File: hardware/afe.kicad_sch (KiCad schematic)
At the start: 53 parts, among them J2 DNP, J3 DNP, J4 Conn_01x19_Male, U2 BQ76200PW, U3 LTC6813-1

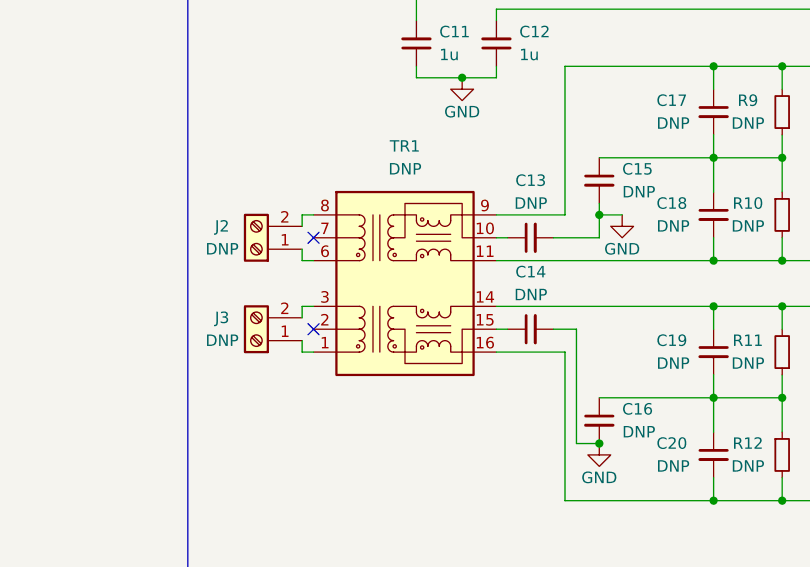
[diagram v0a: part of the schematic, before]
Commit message: Update design to KiCAD v7
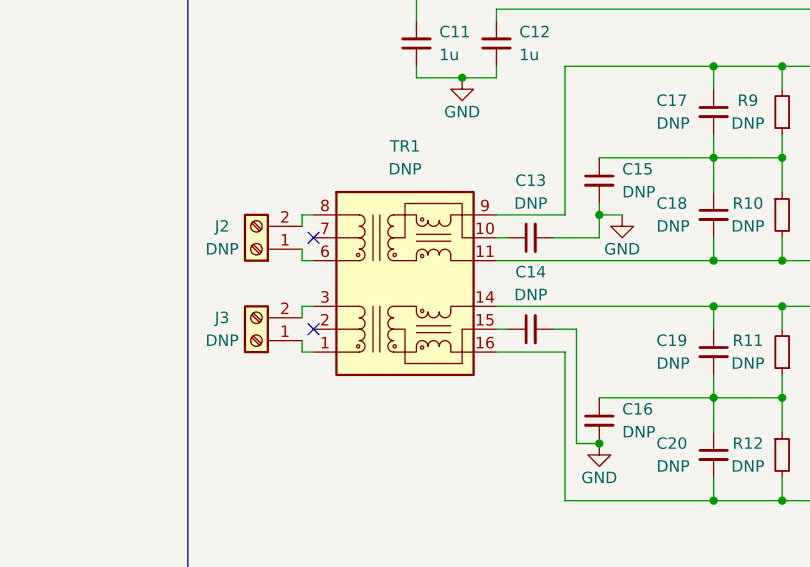
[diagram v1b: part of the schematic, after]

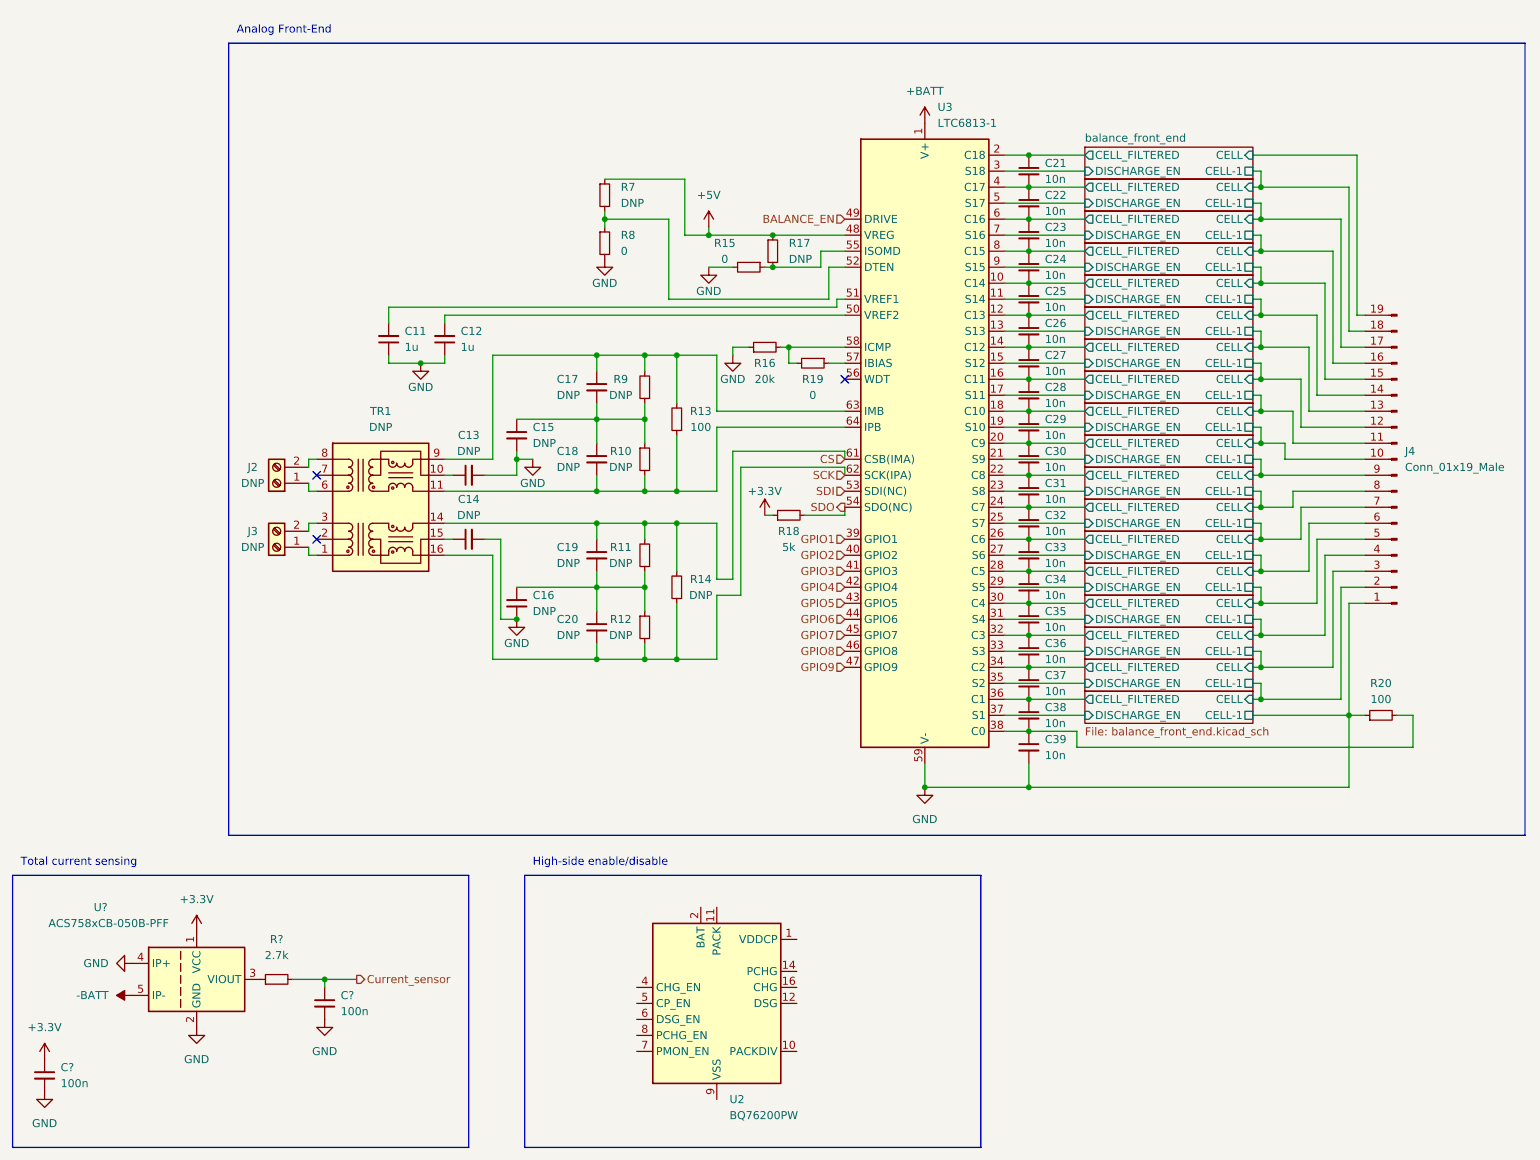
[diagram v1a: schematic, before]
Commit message: DNP marks from new KiCAD
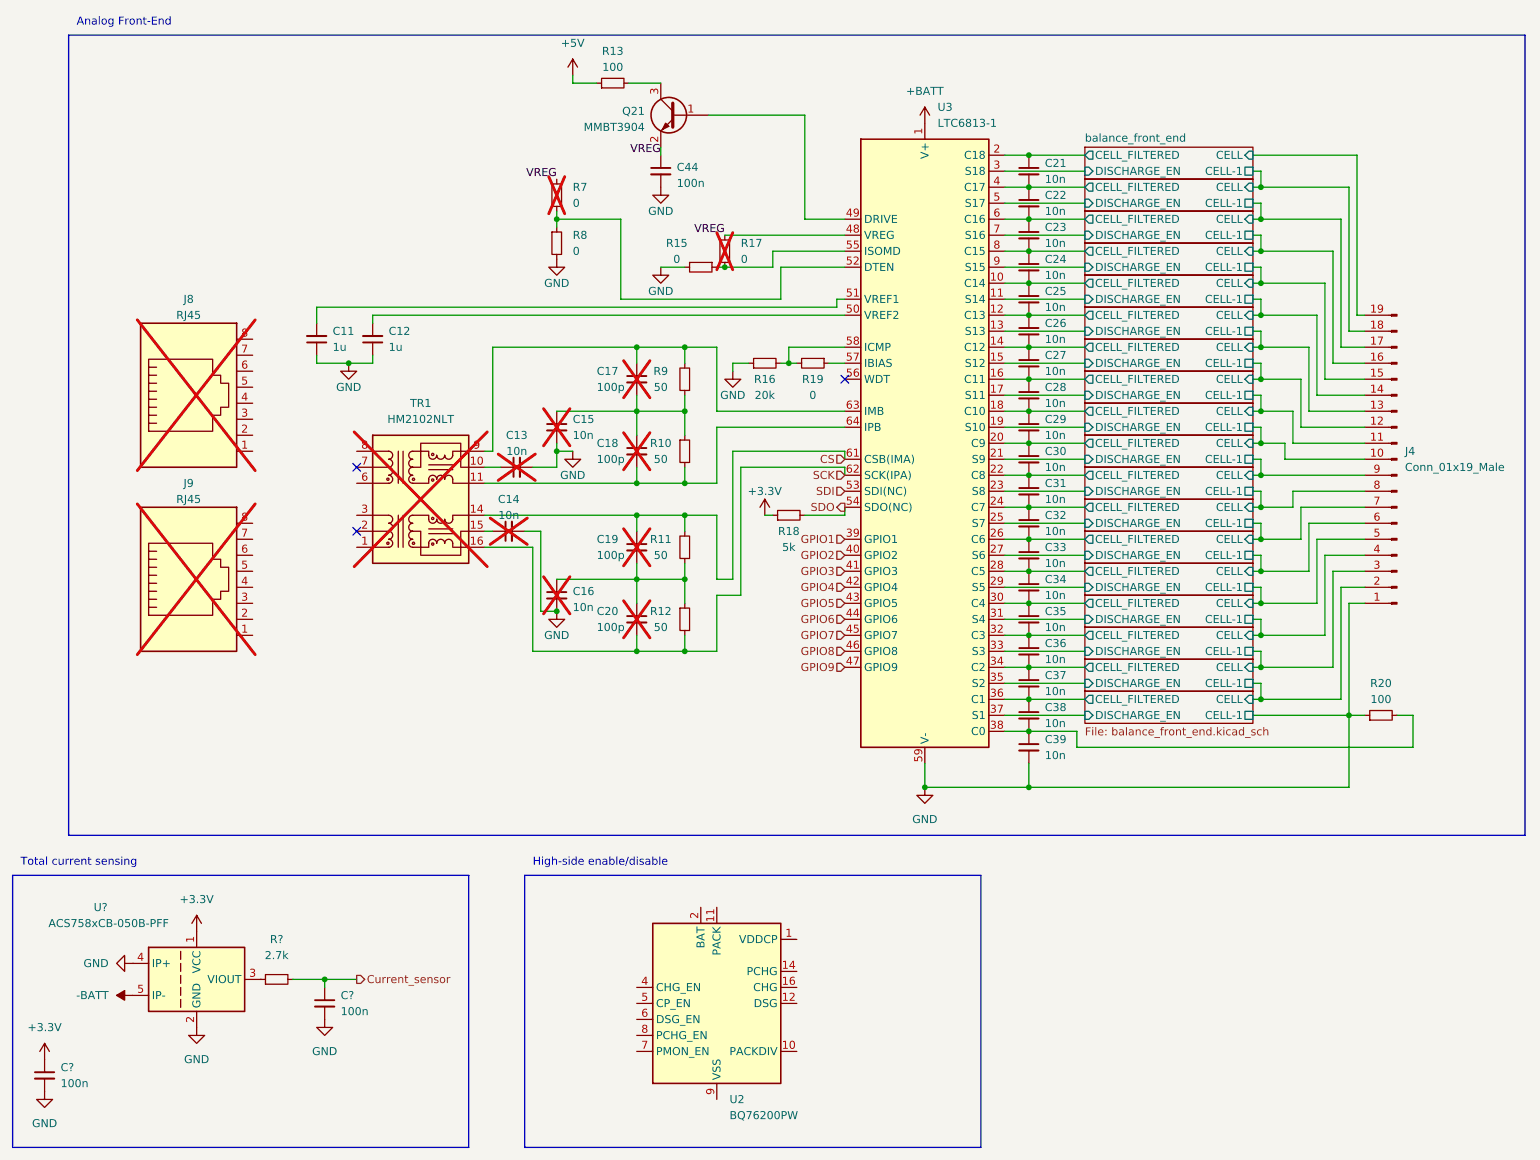
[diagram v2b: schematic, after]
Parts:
- removed J2, J3: DNP, symbol Connector:Screw_Terminal_01x02
- removed R14: DNP, symbol Device:R_Small
- added C44: 100n, symbol Device:C_Small
- added J8, J9: RJ45, symbol Connector:RJ45
- added Q21: MMBT3904, Package_TO_SOT_SMD:SOT-23, symbol Transistor_BJT:MMBT3904
- C13, C14, C15, C16: value DNP -> 10n; now not fitted
- C17, C18, C19, C20: value DNP -> 100p; now not fitted
- R10, R11, R12, R9: value DNP -> 50
- R17, R7: value DNP -> 0; now not fitted
- TR1: value DNP -> HM2102NLT; now not fitted
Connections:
- net +5V: now also R13.1; no longer R17.1, R7.1, U3.48 (VREG)
- net GND: now also C44.2
- net at C17.1, R9.2, TR1.9 (RX-)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: no longer R13.2
- net at C18.2, R10.2, TR1.11 (RX+)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: no longer R13.1
- net BALANCE_EN: no longer names the net of U3.49 (DRIVE)
- net BALANCE_EN: now also Q21.1 (B)
- new net: Q21.3 (C), R13.2
- new net VREG: C44.1, Q21.2 (E), R17.1, R7.1, U3.48 (VREG)
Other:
- moved on the sheet: C11, C12, R10, R11, R12, R15, R16, R8, R9

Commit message: Work on thermal
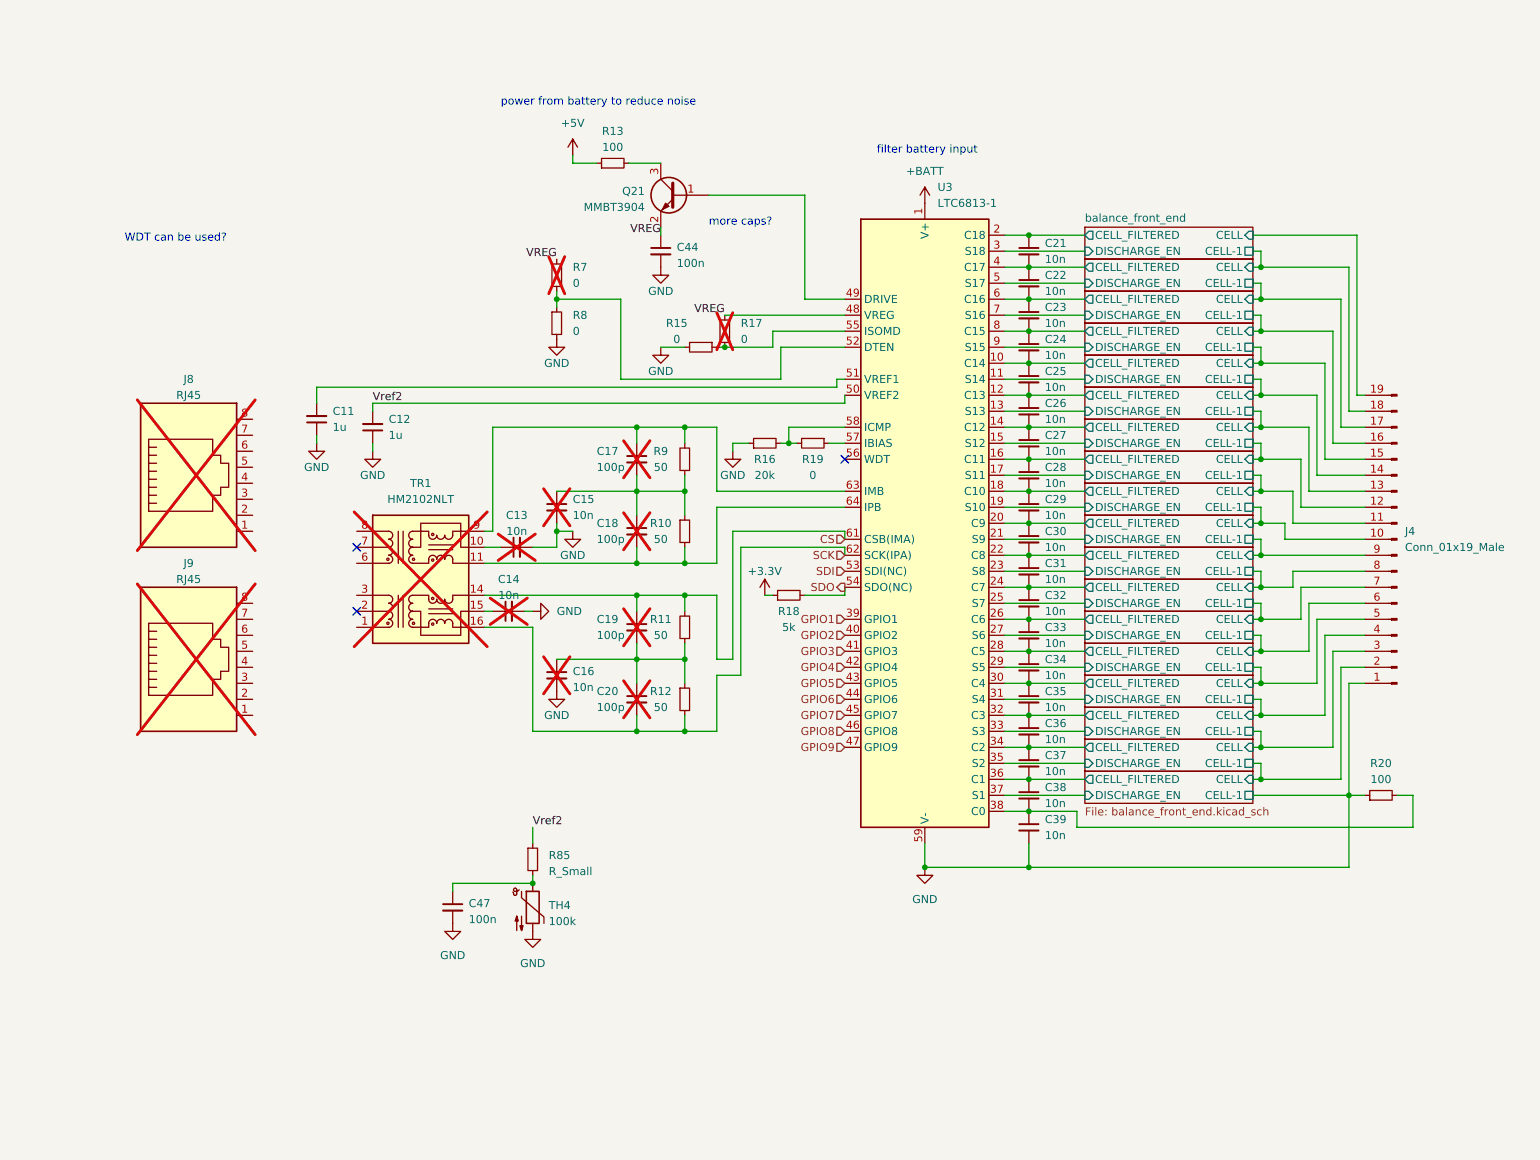
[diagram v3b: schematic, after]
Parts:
- removed C? (x2): 100n, symbol Device:C_Small
- removed R?: 2.7k, symbol Device:R_Small
- removed U2: BQ76200PW, Package_SO:TSSOP-16_4.4x5mm_P0.65mm, symbol Battery_Management:BQ76200PW
- removed U?: ACS758xCB-050B-PFF, Sensor_Current:Allegro_CB_PFF, symbol Sensor_Current:ACS758xCB-050B-PFF
- added C47: 100n, symbol Device:C_Small
- added R85: R_Small, symbol Device:R_Small
- added TH4: 100k, symbol Device:Thermistor_NTC
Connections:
- net GND: now also C47.2, TH4.2
- net Vref2: now reaches C12.2, U3.50 (VREF2)
- net Vref2: now also R85.1
- new net: C47.1, R85.2, TH4.1
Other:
- note added: "WDT can be used?"
- note added: "filter battery input"
- note added: "more caps?"
- note added: "power from battery to reduce noise"
- note removed: "Analog Front-End"
- note removed: "High-side enable/disable"
- note removed: "Total current sensing"
- moved on the sheet: C11, C12, C13, C14, C15, C16, C17, C18, C19, C20, C21, C22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
